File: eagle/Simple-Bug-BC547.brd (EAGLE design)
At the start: 27.9 x 20.3 mm, 14 parts, among them T1 BC547

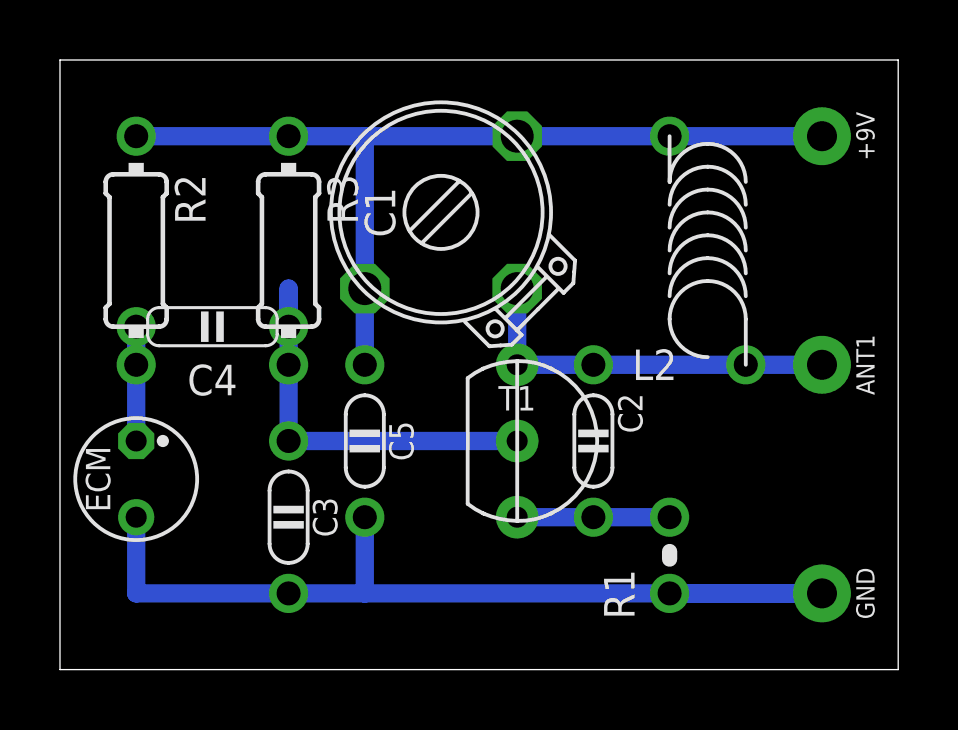
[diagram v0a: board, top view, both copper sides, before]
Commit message: ...
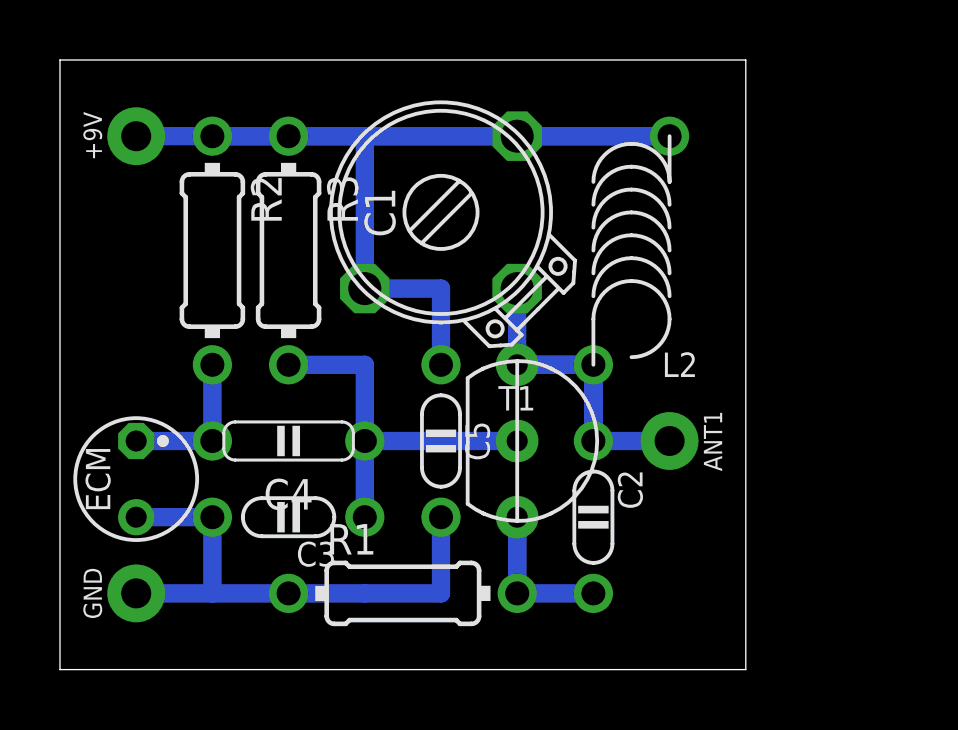
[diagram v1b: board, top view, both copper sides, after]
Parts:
- C3: device c:C050-020X036/V -> c:C050-020X036
- L2: device l:L-04/7V -> l:L-04/7V-X
- R1: device r:0204/2V -> r:0204/7
- moved +9V 22.9 mm to (2.54, 17.8), turned to 0 degrees
- moved GND 22.9 mm to (2.54, 2.54), turned to 0 degrees
- moved R1 8.98 mm to (11.4, 2.54), turned to 0 degrees
- moved ANT1 5.68 mm to (20.3, 7.62)
- moved C4 4.58 mm to (7.62, 7.62)
- moved L2 2.84 mm to (19.1, 14.0)
- moved C2 2.54 mm to (17.8, 5.08)
- moved R2 2.54 mm to (5.08, 14.0)
- moved C5 2.54 mm to (12.7, 7.62)
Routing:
- net GND: track 33.0 -> 17.8 mm
- net +UB: track 30.5 -> 43.2 mm
- net N$2: track 12.7 -> 15.2 mm
- net N$3: track 5.08 -> 7.62 mm
- net N$6: track 3.81 -> 5.08 mm
- net N$5: track 14.0 -> 12.7 mm
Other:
- board size 27.9 x 20.3 mm -> 22.9 x 20.3 mm
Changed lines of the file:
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@@
 <setting verticaltext="up"/>
 </settings>
-<grid distance="0.05" unitdist="inch" unit="inch" style="lines" multiple="2" display="yes" altdistance="10" altunitdist="mil" altunit="inch"/>
+<grid distance="0.05" unitdist="inch" unit="inch" style="dots" multiple="2" display="yes" altdistance="10" altunitdist="mil" altunit="inch"/>
 <layers>
 <layer number="1" name="Top" color="4" fill="1" visible="yes" active="yes"/>
@@
 <description>Simple FM Transmitter with Electret Microphone, based on NPN Transistor</description>
 <plain>
-<wire x1="27.94" y1="0" x2="0" y2="0" width="0" layer="20"/>
+<wire x1="22.86" y1="0" x2="0" y2="0" width="0" layer="20"/>
 <wire x1="0" y1="0" x2="0" y2="20.32" width="0" layer="20"/>
-<wire x1="0" y1="20.32" x2="27.94" y2="20.32" width="0" layer="20"/>
-<wire x1="27.94" y1="20.32" x2="27.94" y2="0" width="0" layer="20"/>
+<wire x1="0" y1="20.32" x2="22.86" y2="20.32" width="0" layer="20"/>
+<wire x1="22.86" y1="20.32" x2="22.86" y2="0" width="0" layer="20"/>
 </plain>
 <attributes>
@@
 </autorouter>
 <elements>
-<element name="C2" library="c" package="C050-020X036" value="4.7pF" x="17.78" y="7.62" smashed="yes" rot="R270">
-<attribute name="NAME" x="18.6055" y="7.874" size="0.8128" layer="25" rot="R270" align="bottom-right"/>
-<attribute name="VALUE" x="16.0655" y="8.636" size="0.8128" layer="27" rot="R270"/>
+<element name="C2" library="c" package="C050-020X036" value="4.7pF" x="17.78" y="5.08" smashed="yes" rot="R270">
+<attribute name="NAME" x="18.6055" y="5.334" size="0.8128" layer="25" rot="R270" align="bottom-right"/>
+<attribute name="VALUE" x="16.0655" y="6.096" size="0.8128" layer="27" rot="R270"/>
 </element>
-<element name="C3" library="c" package="C050-020X036/V" value="1nF" x="7.62" y="5.08" rot="R180"/>
-<element name="R2" library="r" package="0204/7-V" value="4.7k" x="2.54" y="13.97" rot="R180"/>
+<element name="C3" library="c" package="C050-020X036" value="1nF" x="7.62" y="5.08" rot="R180"/>
+<element name="R2" library="r" package="0204/7-V" value="4.7k" x="5.08" y="13.97" rot="R180"/>
 <element name="R3" library="r" package="0204/7-V" value="33k" x="7.62" y="13.97" rot="R180"/>
 <element name="ECM" library="ECM" package="ECM-4" value="ECM-4" x="2.54" y="6.35"/>
 <element name="C1" library="cap-trim" package="TRIM-2222-808" value="1.6-15pF" x="12.7" y="15.24" rot="R90"/>
-<element name="R1" library="r" package="0204/2V" value="4.7" x="20.32" y="3.81" rot="R90"/>
-<element name="C4" library="c" package="C050-020X044" value="330nF" x="5.08" y="11.43" rot="R180"/>
-<element name="+9V" library="pad" package="SPAD" value="SPAD" x="25.4" y="17.78" rot="R180"/>
-<element name="GND" library="pad" package="SPAD" value="SPAD" x="25.4" y="2.54" rot="R180"/>
-<element name="ANT1" library="pad" package="SPAD" value="ANT" x="25.4" y="10.16" rot="R180"/>
-<element name="C5" library="c" package="C050-020X036/V" value="22nF" x="10.16" y="7.62" rot="R180"/>
+<element name="R1" library="r" package="0204/7" value="4.7" x="11.43" y="2.54"/>
+<element name="C4" library="c" package="C050-020X044" value="330nF" x="7.62" y="7.62" rot="R180"/>
+<element name="+9V" library="pad" package="SPAD" value="SPAD" x="2.54" y="17.78"/>
+<element name="GND" library="pad" package="SPAD" value="SPAD" x="2.54" y="2.54"/>
+<element name="ANT1" library="pad" package="SPAD" value="ANT" x="20.32" y="7.62" rot="R180"/>
+<element name="C5" library="c" package="C050-020X036/V" value="22nF" x="12.7" y="7.62" rot="R180"/>
 <element name="T1" library="t" package="TO92-CBE" value="BC547" x="15.24" y="7.62" smashed="yes">
 <attribute name="NAME" x="15.24" y="8.636" size="0.8128" layer="25" ratio="10" rot="R180" align="top-center"/>
 <attribute name="VALUE" x="11.811" y="7.62" size="0.8128" layer="27" ratio="10" rot="R90" align="bottom-center"/>
 </element>
-<element name="L2" library="l" package="L-04/7V" value="1uH" x="21.59" y="15.24"/>
+<element name="L2" library="l" package="L-04/7V-X" value="1uH" x="19.05" y="13.97"/>
 </elements>
 <signals>
@@
 <contactref element="R1" pad="2"/>
 <contactref element="T1" pad="E"/>
-<wire x1="15.24" y1="5.08" x2="17.78" y2="5.08" width="0.6096" layer="16"/>
-<wire x1="20.32" y1="5.08" x2="17.78" y2="5.08" width="0.6096" layer="16"/>
+<wire x1="15.24" y1="5.08" x2="15.24" y2="2.54" width="0.6096" layer="16"/>
+<wire x1="17.78" y1="2.54" x2="15.24" y2="2.54" width="0.6096" layer="16"/>
+<wire x1="15.24" y1="2.54" x2="15.24" y2="5.08" width="0.6096" layer="16"/>
 </signal>
 <signal name="N$5">
@@
 <contactref element="C4" pad="2"/>
 <contactref element="T1" pad="B"/>
-<wire x1="7.62" y1="12.7" x2="7.62" y2="10.16" width="0.6096" layer="16"/>
-<wire x1="7.62" y1="7.62" x2="15.24" y2="7.62" width="0.6096" layer="16"/>
-<wire x1="7.62" y1="10.16" x2="7.62" y2="7.62" width="0.6096" layer="16"/>
-<wire x1="7.62" y1="11.43" x2="7.62" y2="12.7" width="0.6096" layer="16"/>
+<wire x1="10.16" y1="7.62" x2="15.24" y2="7.62" width="0.6096" layer="16"/>
+<wire x1="10.16" y1="5.08" x2="10.16" y2="7.62" width="0.6096" layer="16"/>
+<wire x1="10.16" y1="7.62" x2="10.16" y2="10.16" width="0.6096" layer="16"/>
+<wire x1="10.16" y1="10.16" x2="7.62" y2="10.16" width="0.6096" layer="16"/>
 </signal>
 <signal name="N$6">
@@
 <contactref element="C4" pad="1"/>
 <contactref element="ECM" pad="1"/>
-<wire x1="2.54" y1="7.62" x2="2.54" y2="10.16" width="0.6096" layer="16"/>
-<wire x1="2.54" y1="11.43" x2="2.54" y2="10.16" width="0.6096" layer="16"/>
+<wire x1="2.54" y1="7.62" x2="5.08" y2="7.62" width="0.6096" layer="16"/>
+<wire x1="5.08" y1="7.62" x2="5.08" y2="10.16" width="0.6096" layer="16"/>
 </signal>
 <signal name="GND">
@@
 <contactref element="R1" pad="1"/>
 <contactref element="GND" pad="1"/>
-<wire x1="7.62" y1="2.54" x2="2.54" y2="2.54" width="0.6096" layer="16"/>
-<wire x1="25.4" y1="2.54" x2="10.16" y2="2.54" width="0.6096" layer="16"/>
 <contactref element="C5" pad="2"/>
+<contactref element="ECM" pad="2"/>
+<wire x1="12.7" y1="5.08" x2="12.7" y2="2.54" width="0.6096" layer="16"/>
+<wire x1="12.7" y1="2.54" x2="10.16" y2="2.54" width="0.6096" layer="16"/>
 <wire x1="10.16" y1="2.54" x2="7.62" y2="2.54" width="0.6096" layer="16"/>
-<contactref element="ECM" pad="2"/>
-<wire x1="10.16" y1="5.08" x2="10.16" y2="2.54" width="0.6096" layer="16"/>
-<wire x1="20.32" y1="2.54" x2="25.4" y2="2.54" width="0.6096" layer="16"/>
-<wire x1="2.54" y1="5.08" x2="2.54" y2="2.54" width="0.6096" layer="16"/>
+<wire x1="7.62" y1="2.54" x2="5.08" y2="2.54" width="0.6096" layer="16"/>
+<wire x1="5.08" y1="2.54" x2="5.08" y2="5.08" width="0.6096" layer="16"/>
+<wire x1="5.08" y1="2.54" x2="2.54" y2="2.54" width="0.6096" layer="16"/>
+<wire x1="5.08" y1="5.08" x2="2.54" y2="5.08" width="0.6096" layer="16"/>
 </signal>
 <signal name="+UB">
@@
 <wire x1="10.16" y1="12.7" x2="10.16" y2="17.78" width="0.6096" layer="16"/>
 <wire x1="10.16" y1="17.78" x2="7.62" y2="17.78" width="0.6096" layer="16"/>
-<wire x1="10.16" y1="10.16" x2="10.16" y2="12.7" width="0.6096" layer="16"/>
-<wire x1="2.54" y1="17.78" x2="7.62" y2="17.78" width="0.6096" layer="16"/>
+<wire x1="12.7" y1="10.16" x2="12.7" y2="12.7" width="0.6096" layer="16"/>
+<wire x1="12.7" y1="12.7" x2="10.16" y2="12.7" width="0.6096" layer="16"/>
+<wire x1="5.08" y1="17.78" x2="7.62" y2="17.78" width="0.6096" layer="16"/>
 <contactref element="L2" pad="2"/>
-<wire x1="10.16" y1="17.78" x2="25.4" y2="17.78" width="0.6096" layer="16"/>
-<wire x1="15.24" y1="17.78" x2="20.32" y2="17.78" width="0" layer="19" extent="1-1"/>
-<wire x1="25.4" y1="17.78" x2="20.32" y2="17.78" width="0" layer="19" extent="1-1"/>
+<wire x1="10.16" y1="17.78" x2="15.24" y2="17.78" width="0.6096" layer="16"/>
+<wire x1="15.24" y1="17.78" x2="20.32" y2="17.78" width="0.6096" layer="16"/>
+<wire x1="20.32" y1="17.78" x2="2.54" y2="17.78" width="0.6096" layer="16"/>
 </signal>
 <signal name="N$2">
@@
 <contactref element="ANT1" pad="1"/>
 <contactref element="C1" pad="2"/>
-<wire x1="25.4" y1="10.16" x2="17.78" y2="10.16" width="0.6096" layer="16"/>
+<wire x1="20.32" y1="7.62" x2="17.78" y2="7.62" width="0.6096" layer="16"/>
+<wire x1="17.78" y1="7.62" x2="17.78" y2="10.16" width="0.6096" layer="16"/>
 <wire x1="15.24" y1="10.16" x2="17.78" y2="10.16" width="0.6096" layer="16"/>
+<wire x1="17.78" y1="10.16" x2="17.78" y2="7.62" width="0.6096" layer="16"/>
 <wire x1="15.24" y1="10.16" x2="15.24" y2="12.7" width="0.6096" layer="16"/>
-<wire x1="25.4" y1="10.16" x2="22.86" y2="10.16" width="0" layer="19" extent="1-1"/>
+<wire x1="15.24" y1="10.16" x2="17.78" y2="10.16" width="0.6096" layer="16"/>
 </signal>
 </signals>
